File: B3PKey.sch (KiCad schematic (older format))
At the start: 4 parts

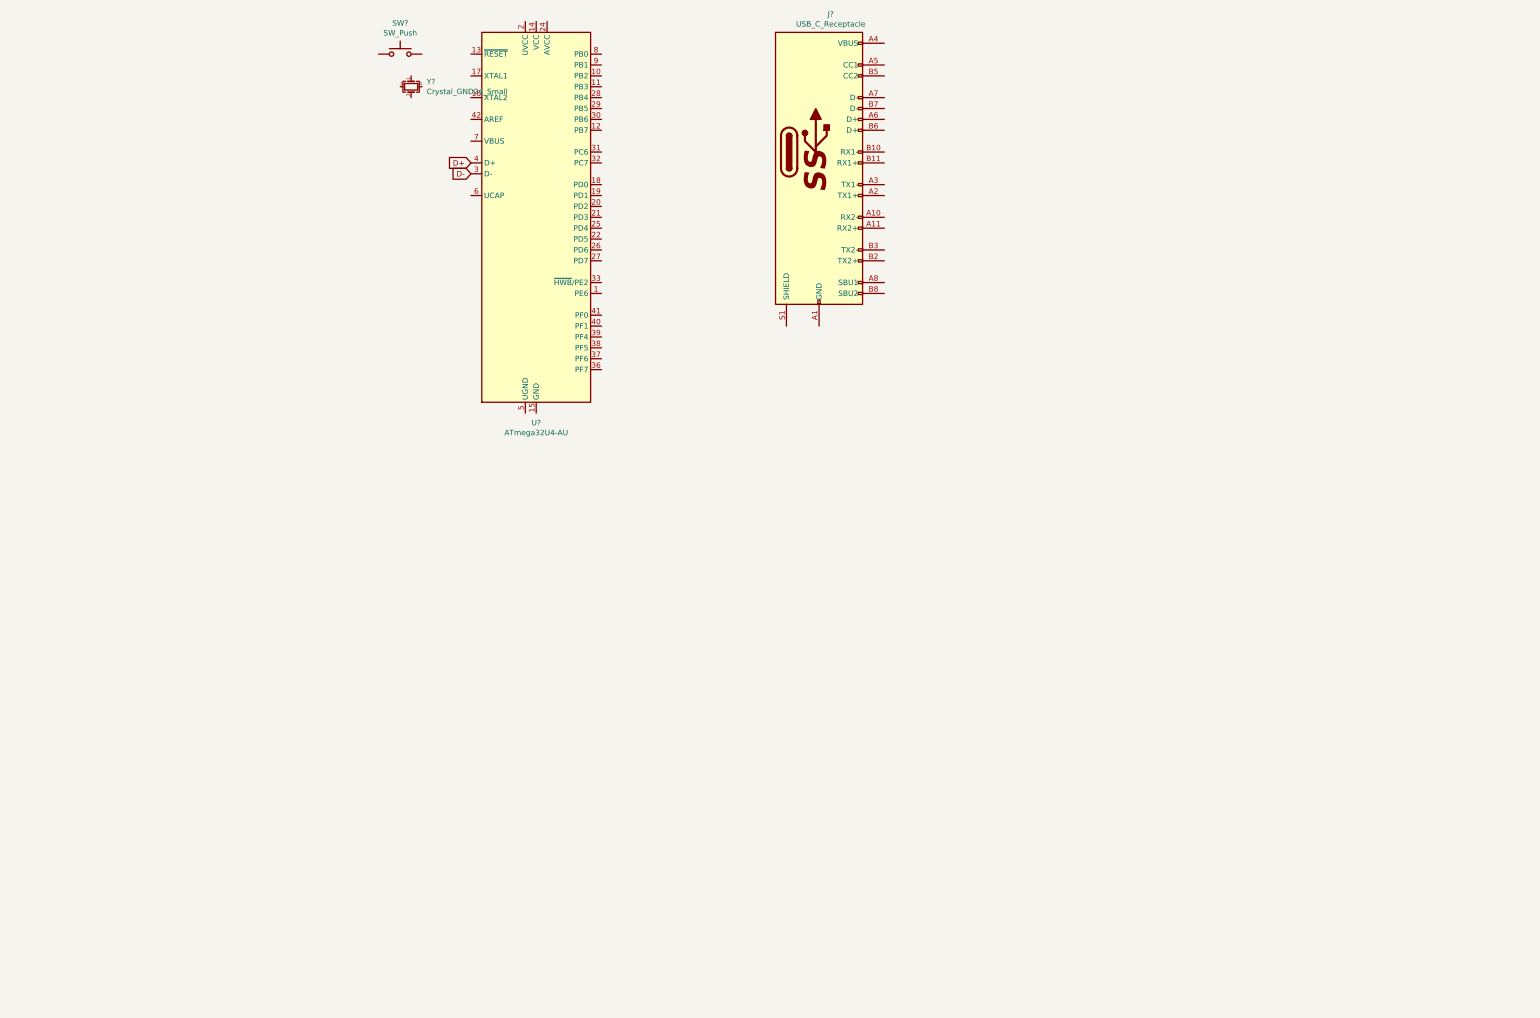
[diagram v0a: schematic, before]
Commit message: Controller and keyswitch schematic
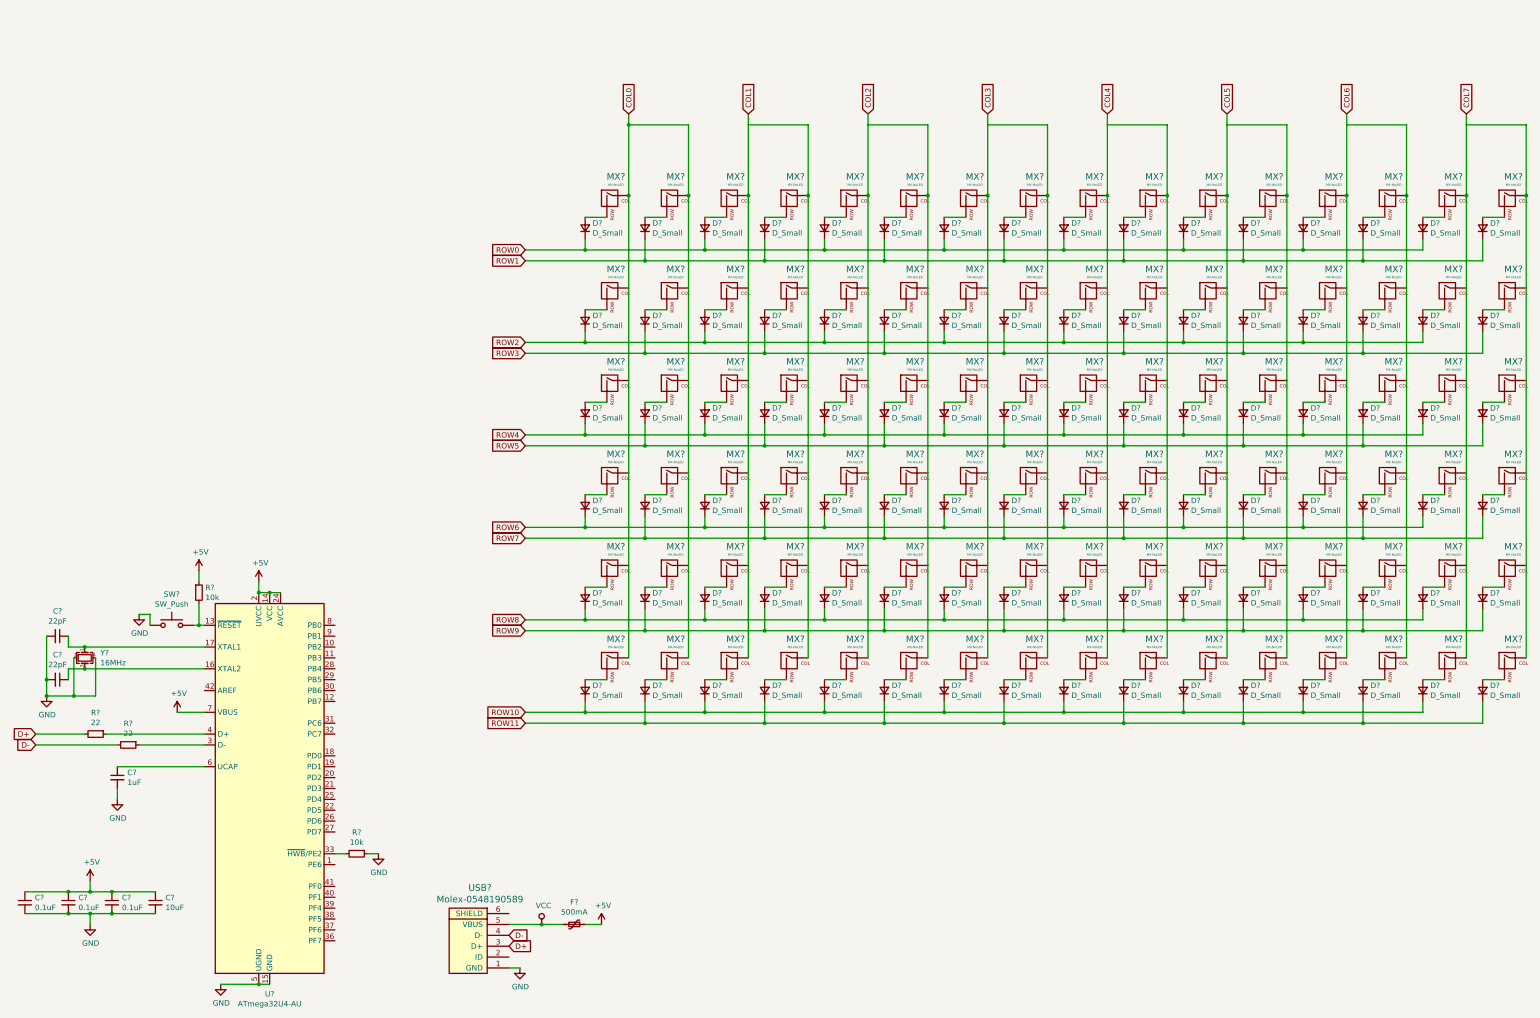
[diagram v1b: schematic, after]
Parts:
- removed J?: USB_C_Receptacle, symbol Connector:USB_C_Receptacle
- added C?: 1uF, symbol Device:C_Small
- added C? (x3): 0.1uF, symbol Device:C_Small
- added C?: 10uF, symbol Device:C_Small
- added C? (x2): 22pF, symbol Device:C_Small
- added D? (x96): D_Small, symbol Device:D_Small
- added F?: 500mA, symbol Device:Polyfuse_Small
- added MX? (x96): MX-NoLED, symbol MX_Alps_Hybrid:MX-NoLED
- added R? (x2): 10k, symbol Device:R_Small
- added R? (x2): 22, symbol Device:R_Small
- added USB?: Molex-0548190589, symbol random-keyboard-parts:Molex-0548190589
- Y?: value Crystal_GND24_Small -> 16MHz
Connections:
- net D+: now also R?.2, USB?.3 (D+); no longer U?.4 (D+)
- net D-: now also R?.2, USB?.4 (D-); no longer U?.3 (D-)
- net at U?.13 (~RESET): now also SW?.2, R?.2
- net +5V: now reaches U?.14 (VCC), U?.34 (VCC)
- net +5V: now also U?.2 (UVCC), U?.24 (AVCC), U?.44 (AVCC), U?.7 (VBUS), C?.1, C?.1, C?.1, C?.1, F?.1, R?.1
- net GND: now reaches U?.15 (GND), U?.23 (GND), U?.35 (GND), U?.43 (GND)
- net GND: now also SW?.1, U?.5 (UGND), Y?.2, Y?.4, C?.2, C?.2, C?.2, C?.2, C?.2, C?.2, C?.2, R?.1, USB?.1 (GND)
- net at U?.16 (XTAL2): now also Y?.3, C?.1
- net at U?.17 (XTAL1): now also Y?.1, C?.1
- net at U?.33 (~HWB~/PE2): now also R?.2
- net at U?.6 (UCAP): now also C?.1
- new net: R?.1, U?.3 (D-)
- new net: R?.1, U?.4 (D+)
- new net: D?.2 (A), MX?.2 (ROW) (x96)
- new net COL0: MX?.1 (COL), MX?.1 (COL), MX?.1 (COL), MX?.1 (COL), MX?.1 (COL), MX?.1 (COL), MX?.1 (COL), MX?.1 (COL), MX?.1 (COL), MX?.1 (COL), MX?.1 (COL), MX?.1 (COL)
- new net COL1: MX?.1 (COL), MX?.1 (COL), MX?.1 (COL), MX?.1 (COL), MX?.1 (COL), MX?.1 (COL), MX?.1 (COL), MX?.1 (COL), MX?.1 (COL), MX?.1 (COL), MX?.1 (COL), MX?.1 (COL)
- new net COL2: MX?.1 (COL), MX?.1 (COL), MX?.1 (COL), MX?.1 (COL), MX?.1 (COL), MX?.1 (COL), MX?.1 (COL), MX?.1 (COL), MX?.1 (COL), MX?.1 (COL), MX?.1 (COL), MX?.1 (COL)
- new net COL3: MX?.1 (COL), MX?.1 (COL), MX?.1 (COL), MX?.1 (COL), MX?.1 (COL), MX?.1 (COL), MX?.1 (COL), MX?.1 (COL), MX?.1 (COL), MX?.1 (COL), MX?.1 (COL), MX?.1 (COL)
- new net COL4: MX?.1 (COL), MX?.1 (COL), MX?.1 (COL), MX?.1 (COL), MX?.1 (COL), MX?.1 (COL), MX?.1 (COL), MX?.1 (COL), MX?.1 (COL), MX?.1 (COL), MX?.1 (COL), MX?.1 (COL)
- new net COL5: MX?.1 (COL), MX?.1 (COL), MX?.1 (COL), MX?.1 (COL), MX?.1 (COL), MX?.1 (COL), MX?.1 (COL), MX?.1 (COL), MX?.1 (COL), MX?.1 (COL), MX?.1 (COL), MX?.1 (COL)
- new net COL6: MX?.1 (COL), MX?.1 (COL), MX?.1 (COL), MX?.1 (COL), MX?.1 (COL), MX?.1 (COL), MX?.1 (COL), MX?.1 (COL), MX?.1 (COL), MX?.1 (COL), MX?.1 (COL), MX?.1 (COL)
- new net COL7: MX?.1 (COL), MX?.1 (COL), MX?.1 (COL), MX?.1 (COL), MX?.1 (COL), MX?.1 (COL), MX?.1 (COL), MX?.1 (COL), MX?.1 (COL), MX?.1 (COL), MX?.1 (COL), MX?.1 (COL)
- new net ROW0: D?.1 (K), D?.1 (K), D?.1 (K), D?.1 (K), D?.1 (K), D?.1 (K), D?.1 (K), D?.1 (K)
- new net ROW1: D?.1 (K), D?.1 (K), D?.1 (K), D?.1 (K), D?.1 (K), D?.1 (K), D?.1 (K), D?.1 (K)
- new net ROW10: D?.1 (K), D?.1 (K), D?.1 (K), D?.1 (K), D?.1 (K), D?.1 (K), D?.1 (K), D?.1 (K)
- new net ROW11: D?.1 (K), D?.1 (K), D?.1 (K), D?.1 (K), D?.1 (K), D?.1 (K), D?.1 (K), D?.1 (K)
- new net ROW2: D?.1 (K), D?.1 (K), D?.1 (K), D?.1 (K), D?.1 (K), D?.1 (K), D?.1 (K), D?.1 (K)
- new net ROW3: D?.1 (K), D?.1 (K), D?.1 (K), D?.1 (K), D?.1 (K), D?.1 (K), D?.1 (K), D?.1 (K)
- new net ROW4: D?.1 (K), D?.1 (K), D?.1 (K), D?.1 (K), D?.1 (K), D?.1 (K), D?.1 (K), D?.1 (K)
- new net ROW5: D?.1 (K), D?.1 (K), D?.1 (K), D?.1 (K), D?.1 (K), D?.1 (K), D?.1 (K), D?.1 (K)
- new net ROW6: D?.1 (K), D?.1 (K), D?.1 (K), D?.1 (K), D?.1 (K), D?.1 (K), D?.1 (K), D?.1 (K)
- new net ROW7: D?.1 (K), D?.1 (K), D?.1 (K), D?.1 (K), D?.1 (K), D?.1 (K), D?.1 (K), D?.1 (K)
- new net ROW8: D?.1 (K), D?.1 (K), D?.1 (K), D?.1 (K), D?.1 (K), D?.1 (K), D?.1 (K), D?.1 (K)
- new net ROW9: D?.1 (K), D?.1 (K), D?.1 (K), D?.1 (K), D?.1 (K), D?.1 (K), D?.1 (K), D?.1 (K)
- new net VCC: F?.2, USB?.5 (VBUS)
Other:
- moved on the sheet: SW?, U?, Y?
